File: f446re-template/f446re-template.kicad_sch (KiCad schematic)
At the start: 21 parts, among them J1 Conn_01x06_Pin, SW1 SW_Push, U1 STM32F446RETx, Y1 16MHz, Y2 32.768KHz

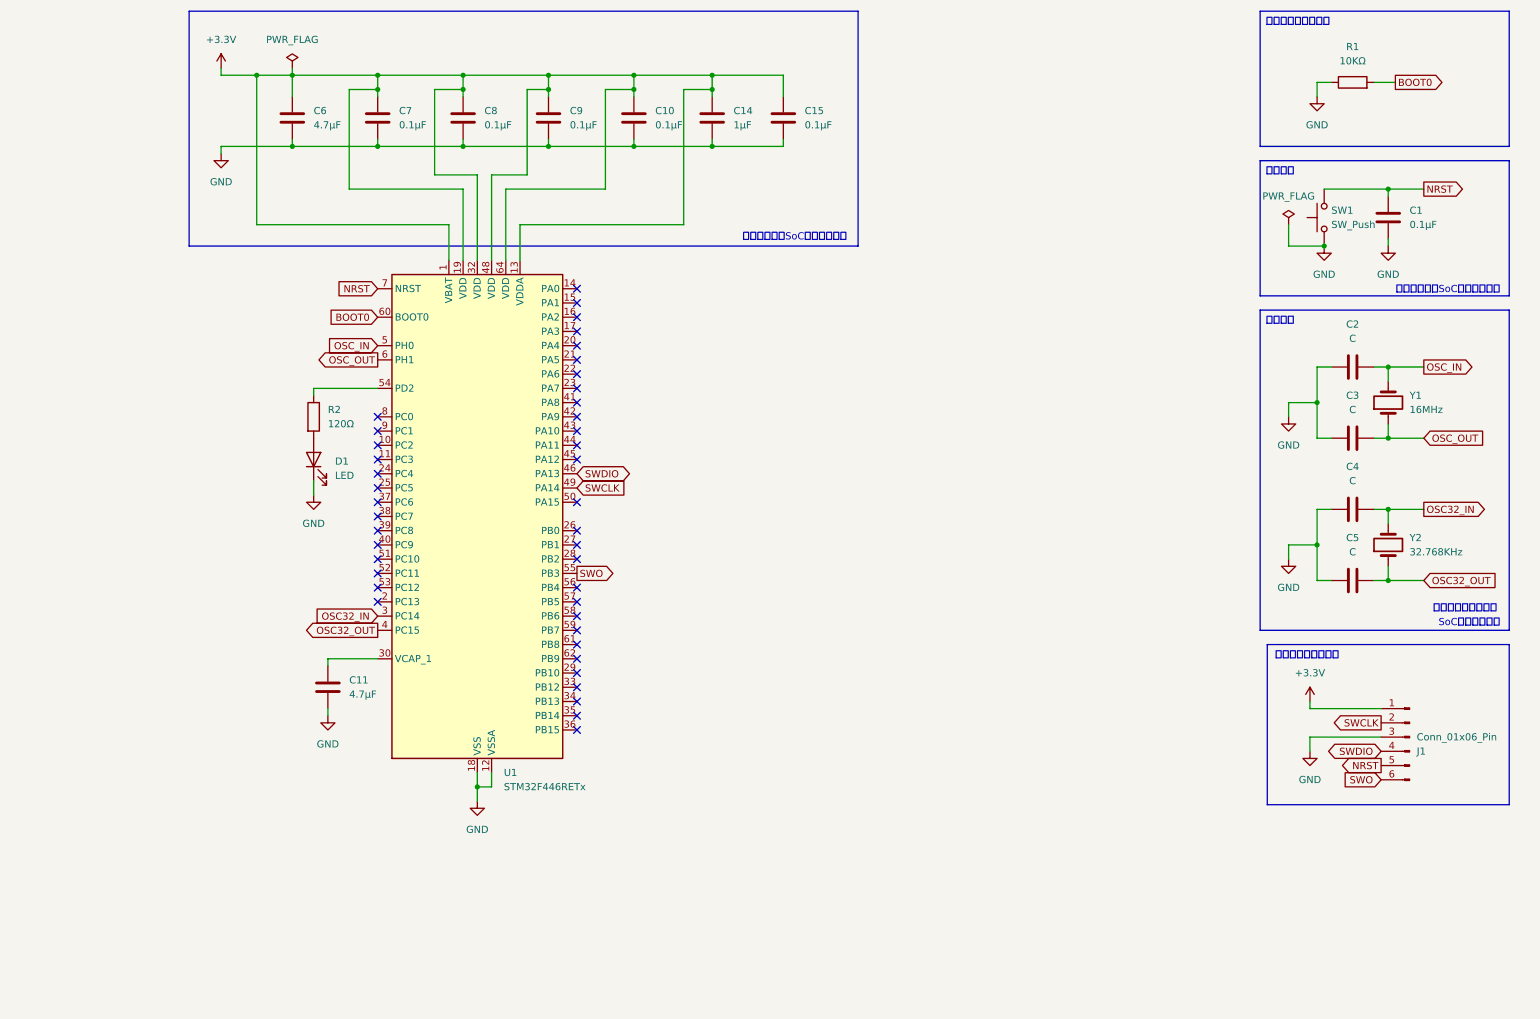
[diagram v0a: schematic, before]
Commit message: 2025/01/31/21:22
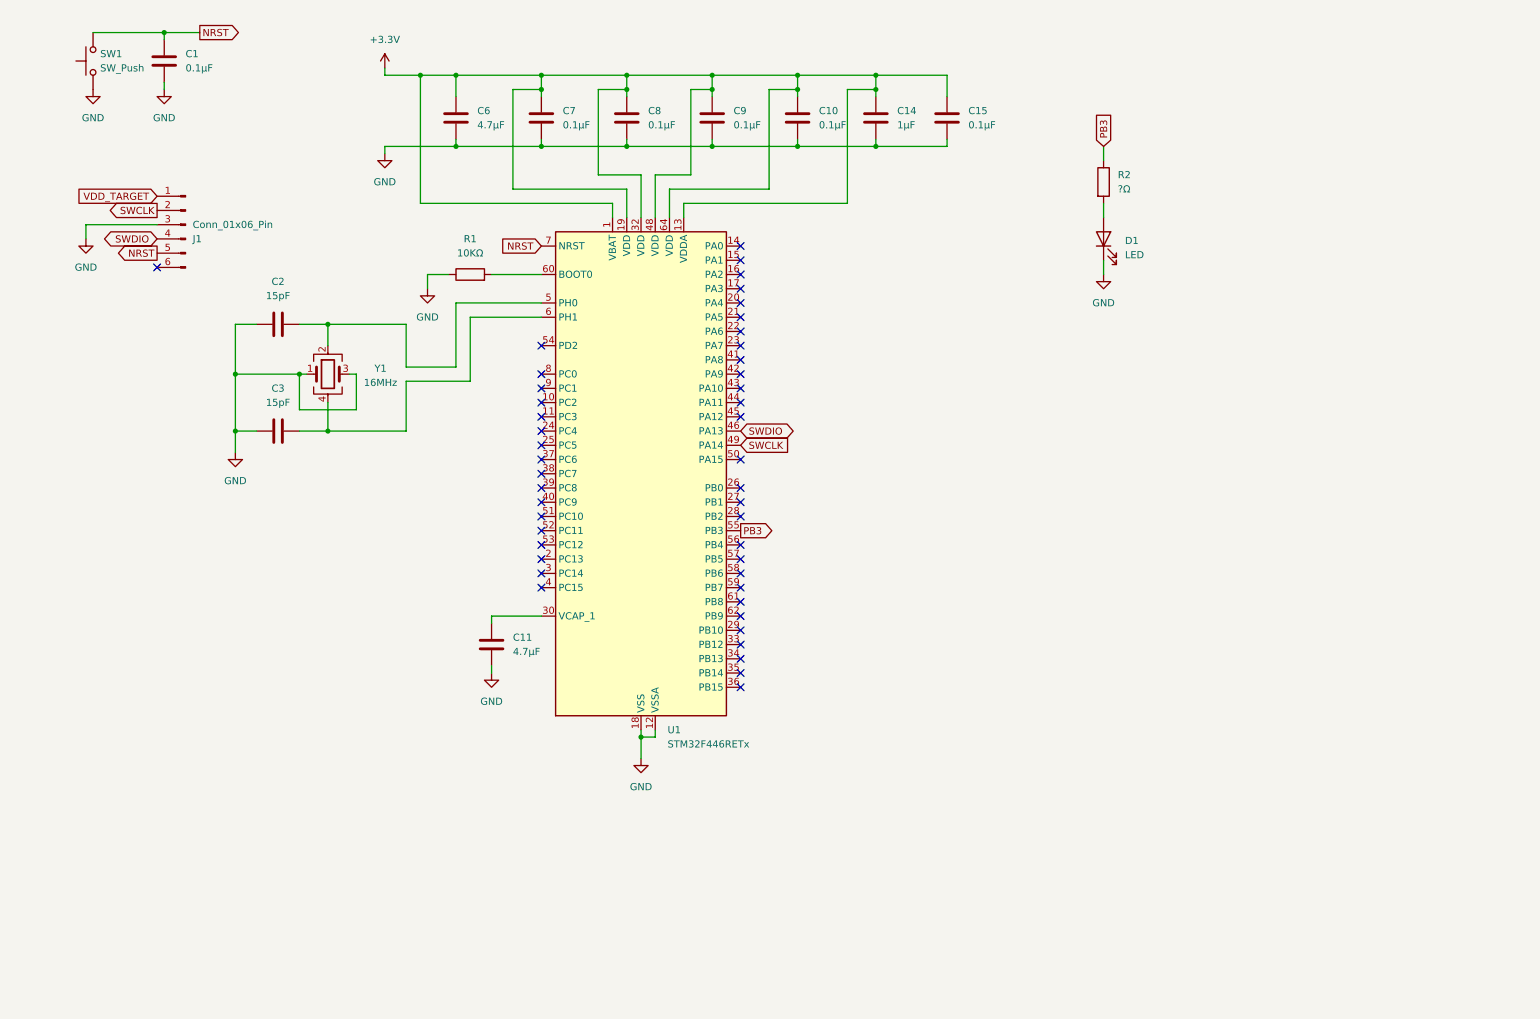
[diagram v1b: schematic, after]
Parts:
- removed C4, C5: C, symbol Device:C
- removed Y1: 16MHz, symbol Device:Crystal
- removed Y2: 32.768KHz, symbol Device:Crystal
- added Y1: 16MHz, Crystal:Crystal_SMD_SeikoEpson_FA238-4Pin_3.2x2.5mm, symbol Device:Crystal_GND24
- C1, C10, C11, C14, C15, C6, C7, C8, C9, R1: footprint (none) -> Capacitor_SMD:C_0603_1608Metric
- C2, C3: value C -> 15pF; footprint (none) -> Capacitor_SMD:C_0603_1608Metric
- D1: footprint (none) -> LED_SMD:LED_0603_1608Metric
- J1: footprint (none) -> Connector_PinSocket_2.54mm:PinSocket_1x06_P2.54mm_Vertical
- R2: value 120Ω -> ?Ω; footprint (none) -> Resistor_SMD:R_0603_1608Metric
- SW1: footprint (none) -> Button_Switch_THT:SW_PUSH_6mm_H5mm
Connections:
- net +3.3V: no longer J1.1 (Pin_1)
- net GND: now also Y1.1, Y1.3
- net at U1.54 (PD2): no longer R2.1
- net BOOT0: no longer names the net of R1.2, U1.60 (BOOT0)
- net OSC32_IN: no longer names the net of U1.3 (PC14)
- net OSC32_OUT: no longer names the net of U1.4 (PC15)
- net OSC_IN: no longer names the net of C2.2, U1.5 (PH0)
- net OSC_IN: now also Y1.2
- net OSC_OUT: no longer names the net of C3.2, U1.6 (PH1)
- net OSC_OUT: now also Y1.4
- net SWO: no longer names the net of J1.6 (Pin_6)
- net SWO: no longer U1.55 (PB3)
- new net PB3: R2.1, U1.55 (PB3)
- new net VDD_TARGET: J1.1 (Pin_1)
- no-connect marks 42 -> 46
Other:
- note removed: "SoCの近くに置く"
- note removed: "コンデンサはSoCの近くに置く"
- note removed: "デバッグ用コネクタ"
- note removed: "配線長を同じにする"
- moved on the sheet: C1, C10, C11, C14, C15, C2, C3, C6, C7, C8, C9, J1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

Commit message: 2025/02/03/12:25
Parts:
- removed C1, C10, C15, C7, C8, C9: 0.1μF, Capacitor_SMD:C_0603_1608Metric, symbol Device:C
- removed C11, C6: 4.7μF, Capacitor_SMD:C_0603_1608Metric, symbol Device:C
- removed C14: 1μF, Capacitor_SMD:C_0603_1608Metric, symbol Device:C
- removed C2, C3: 15pF, Capacitor_SMD:C_0603_1608Metric, symbol Device:C
- removed D1: LED, LED_SMD:LED_0603_1608Metric, symbol Device:LED
- removed J1: Conn_01x06_Pin, Connector_PinSocket_2.54mm:PinSocket_1x06_P2.54mm_Vertical, symbol Connector:Conn_01x06_Pin
- removed R1: 10KΩ, Capacitor_SMD:C_0603_1608Metric, symbol Device:R
- removed R2: ?Ω, Resistor_SMD:R_0603_1608Metric, symbol Device:R
- removed SW1: SW_Push, Button_Switch_THT:SW_PUSH_6mm_H5mm, symbol Switch:SW_Push
- removed U1: STM32F446RETx, Package_QFP:LQFP-64_10x10mm_P0.5mm, symbol MCU_ST_STM32F4:STM32F446RETx
- removed Y1: 16MHz, Crystal:Crystal_SMD_SeikoEpson_FA238-4Pin_3.2x2.5mm, symbol Device:Crystal_GND24
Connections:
- no-connect marks 46 -> 0

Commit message: 2025/02/08/18:16
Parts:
- added C1: 10uF, Capacitor_SMD:C_0603_1608Metric, symbol Device:C
- added C10, C14, C15, C4, C5, C6, C7, C8: 0.1uF, Capacitor_SMD:C_0603_1608Metric, symbol Device:C
- added C11, C3: 4.7uF, Capacitor_SMD:C_0603_1608Metric, symbol Device:C
- added C12, C13: 15pF, Capacitor_SMD:C_0603_1608Metric, symbol Device:C
- added C2: 22uF, Capacitor_SMD:C_0603_1608Metric, symbol Device:C
- added C9: 1uF, Capacitor_SMD:C_0603_1608Metric, symbol Device:C
- added D1, D2, D3: LED, LED_SMD:LED_0603_1608Metric, symbol Device:LED
- added H1, H2, H3, H4: MountingHole, MountingHole:MountingHole_3.2mm_M3, symbol Mechanical:MountingHole
- added J1: 電源コネクタ, Connector_AMASS:AMASS_XT30PW-M_1x02_P2.50mm_Horizontal, symbol Connector:Conn_01x02_Socket
- added J2: デバッグ端子, Connector_PinSocket_2.54mm:PinSocket_1x05_P2.54mm_Horizontal, symbol Connector:Conn_01x05_Pin
- added J3: CANコネクタ, Connector_JST:JST_XH_S2B-XH-A_1x02_P2.50mm_Horizontal, symbol Connector:Conn_01x02_Socket
- added R1: ???Ω, Resistor_SMD:R_0603_1608Metric, symbol Device:R
- added R2, R3: 200Ω, Resistor_SMD:R_0603_1608Metric, symbol Device:R
- added R4: 10kΩ, Resistor_SMD:R_0603_1608Metric, symbol Device:R
- added R5, R6: 1kΩ, Resistor_SMD:R_0603_1608Metric, symbol Device:R
- added SW1: リセットスイッチ, Button_Switch_THT:SW_PUSH_6mm_H5mm, symbol Switch:SW_Push
- added U1: AZ1117-3.3, Package_TO_SOT_SMD:SOT-223-3_TabPin2, symbol Regulator_Linear:AZ1117-3.3
- added U2: STM32F446RETx, Package_QFP:LQFP-64_10x10mm_P0.5mm, symbol MCU_ST_STM32F4:STM32F446RETx
- added U3: MCP2562-E-SN, Package_SO:SOIC-8_3.9x4.9mm_P1.27mm, symbol Interface_CAN_LIN:MCP2562-E-SN
- added Y1: 16MHz, Crystal:Crystal_HC49-4H_Vertical, symbol Device:Crystal
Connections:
- new net: D3.2 (A), R3.2
- new net: C11.2, U2.30 (VCAP_1)
- new net: C12.2, U2.5 (PH0), Y1.2
- new net: C13.2, U2.6 (PH1), Y1.1
- new net: D2.2 (A), R2.2
- new net: J2.4 (Pin_4), R6.1
- new net: D1.2 (A), R1.2
- new net: J2.2 (Pin_2), R5.1
- new net +3.3V: C15.1, C2.1, C3.1, C4.1, C5.1, C6.1, C7.1, C8.1, C9.1, J2.1 (Pin_1), U1.2 (VO), U2.1 (VBAT), U2.13 (VDDA), U2.19 (VDD), U2.32 (VDD), U2.48 (VDD), U2.64 (VDD), U3.5 (Vio)
- new net +5V: C1.1, C14.2, J1.2 (Pin_2), R1.1, U1.3 (VI), U3.3 (VDD)
- new net BOOT0: R4.2, U2.60 (BOOT0)
- new net CAN+: J3.2 (Pin_2), U3.7 (CANH)
- new net CAN-: J3.1 (Pin_1), U3.6 (CANL)
- new net CAN_RX: U2.61 (PB8), U3.4 (RXD)
- new net CAN_RX_LED: R3.1, U2.15 (PA1)
- new net CAN_TX: U2.62 (PB9), U3.1 (TXD)
- new net CAN_TX_LED: R2.1, U2.14 (PA0)
- new net GND: C1.2, C10.2, C11.1, C12.1, C13.1, C14.1, C15.2, C2.2, C3.2, C4.2, C5.2, C6.2, C7.2, C8.2, C9.2, D1.1 (K), D2.1 (K), D3.1 (K), J1.1 (Pin_1), J2.3 (Pin_3), R4.1, SW1.1, U1.1 (GND), U2.12 (VSSA), U2.18 (VSS), U2.31 (VSS), U2.47 (VSS), U2.63 (VSS), U3.2 (VSS), U3.8 (STBY)
- new net NRST: C10.1, J2.5 (Pin_5), SW1.2, U2.7 (NRST)
- new net SWCLK: R5.2, U2.49 (PA14)
- new net SWDIO: R6.2, U2.46 (PA13)
- no-connect marks 0 -> 7
